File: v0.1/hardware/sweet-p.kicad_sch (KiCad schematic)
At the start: 41 parts, among them J1 Screw_Terminal_01x03, J10 Conn_01x04_Socket, J2 Screw_Terminal_01x02, J3 Conn_01x04_Female, J4 Conn_01x04_Socket, J5 Conn_01x06_Socket, J6 Conn_01x02_Socket, J7 Screw_Terminal_01x04, J8 Conn_01x04_Socket, J9 Conn_01x08_Socket, SW1 SW_Push, U1 adafruit_tpl511x

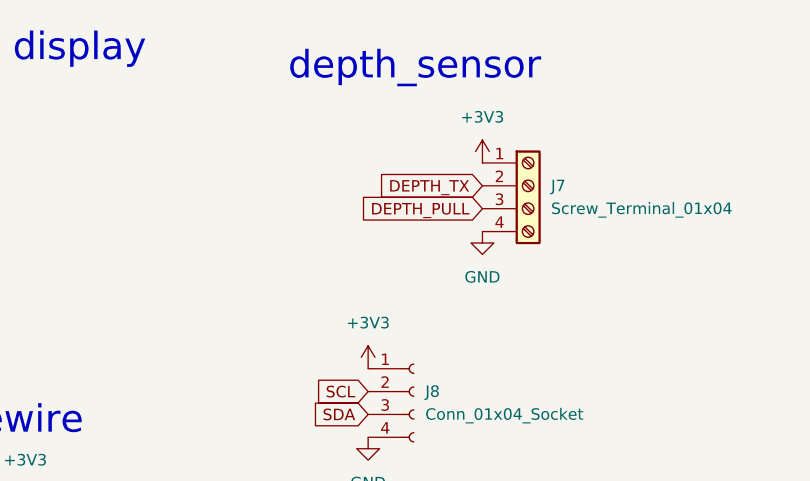
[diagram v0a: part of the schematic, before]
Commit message: update
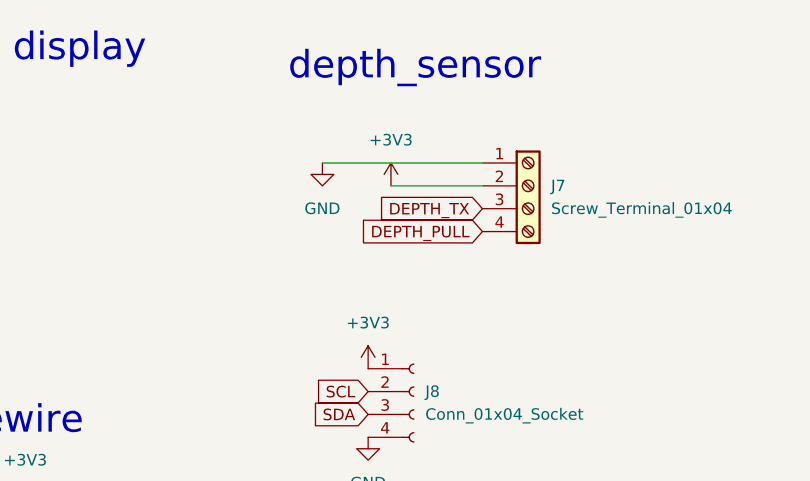
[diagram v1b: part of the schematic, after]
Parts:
- J10: footprint footprints:ssd1306_b -> footprints:ssd1306_a
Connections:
- net +3V3: now also J7.2 (Pin_2); no longer J7.1 (Pin_1)
- net DEPTH_PULL: now also J7.4 (Pin_4); no longer J7.3 (Pin_3)
- net DEPTH_TX: now also J7.3 (Pin_3); no longer J7.2 (Pin_2)
- net GND: now also J7.1 (Pin_1); no longer J7.4 (Pin_4)
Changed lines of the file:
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@@
 	(wire
 		(pts
+			(xy 292.1 33.02) (xy 302.26 33.02)
+		)
+		(stroke
+			(width 0)
+			(type default)
+		)
+	)
+	(wire
+		(pts
 			(xy 133.35 118.11) (xy 142.24 118.11)
 		)
@@
 	(wire
 		(pts
+			(xy 284.48 30.48) (xy 302.26 30.48)
+		)
+		(stroke
+			(width 0)
+			(type default)
+		)
+	)
+	(wire
+		(pts
 			(xy 31.75 95.25) (xy 38.1 95.25)
 		)
@@
 	(global_label "DEPTH_TX"
 		(shape input)
-		(at 302.26 33.02 180)
+		(at 302.26 35.56 180)
 		(fields_autoplaced yes)
 		(effects
@@
 		)
 		(property "Intersheetrefs" "${INTERSHEET_REFS}"
-			(at 290.143 33.02 0)
+			(at 290.143 35.56 0)
 			(effects
 				(font
@@
 	(global_label "DEPTH_PULL"
 		(shape input)
-		(at 302.26 35.56 180)
+		(at 302.26 38.1 180)
 		(fields_autoplaced yes)
 		(effects
@@
 		)
 		(property "Intersheetrefs" "${INTERSHEET_REFS}"
-			(at 287.6634 35.56 0)
+			(at 287.6634 38.1 0)
 			(effects
 				(font
@@
 	(symbol
 		(lib_id "power:+3V3")
-		(at 302.26 30.48 0)
+		(at 292.1 33.02 0)
 		(unit 1)
 		(exclude_from_sim no)
@@
 		(fields_autoplaced yes)
 		(property "Reference" "#PWR030"
-			(at 302.26 34.29 0)
+			(at 292.1 36.83 0)
 			(effects
 				(font
@@
 		)
 		(property "Value" "+3V3"
-			(at 302.26 25.4 0)
+			(at 292.1 27.94 0)
 			(effects
 				(font
@@
 		)
 		(property "Footprint" ""
-			(at 302.26 30.48 0)
+			(at 292.1 33.02 0)
 			(effects
 				(font
@@
 		)
 		(property "Datasheet" ""
-			(at 302.26 30.48 0)
+			(at 292.1 33.02 0)
 			(effects
 				(font
@@
 		)
 		(property "Description" ""
-			(at 302.26 30.48 0)
+			(at 292.1 33.02 0)
 			(effects
 				(font
@@
 			)
 		)
-		(property "Footprint" "footprints:ssd1306_b"
+		(property "Footprint" "footprints:ssd1306_a"
 			(at 214.63 24.13 0)
 			(effects
@@
 		(lib_name "GND_11")
 		(lib_id "power:GND")
-		(at 302.26 38.1 0)
+		(at 284.48 30.48 0)
 		(unit 1)
 		(exclude_from_sim no)
@@
 		(fields_autoplaced yes)
 		(property "Reference" "#PWR029"
-			(at 302.26 44.45 0)
+			(at 284.48 36.83 0)
 			(effects
 				(font
@@
 		)
 		(property "Value" "GND"
-			(at 302.26 43.18 0)
+			(at 284.48 35.56 0)
 			(effects
 				(font
@@
 		)
 		(property "Footprint" ""
-			(at 302.26 38.1 0)
+			(at 284.48 30.48 0)
 			(effects
 				(font
@@
 		)
 		(property "Datasheet" ""
-			(at 302.26 38.1 0)
+			(at 284.48 30.48 0)
 			(effects
 				(font
@@
 		)
 		(property "Description" ""
-			(at 302.26 38.1 0)
+			(at 284.48 30.48 0)
 			(effects
 				(font
